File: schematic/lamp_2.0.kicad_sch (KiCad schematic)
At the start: 18 parts, among them J1 220V, J2 Disco lamp, J3 Edison lamp, Q1 BTA16, U1 EL814, U2 MOC3021, U4 TSOP31238

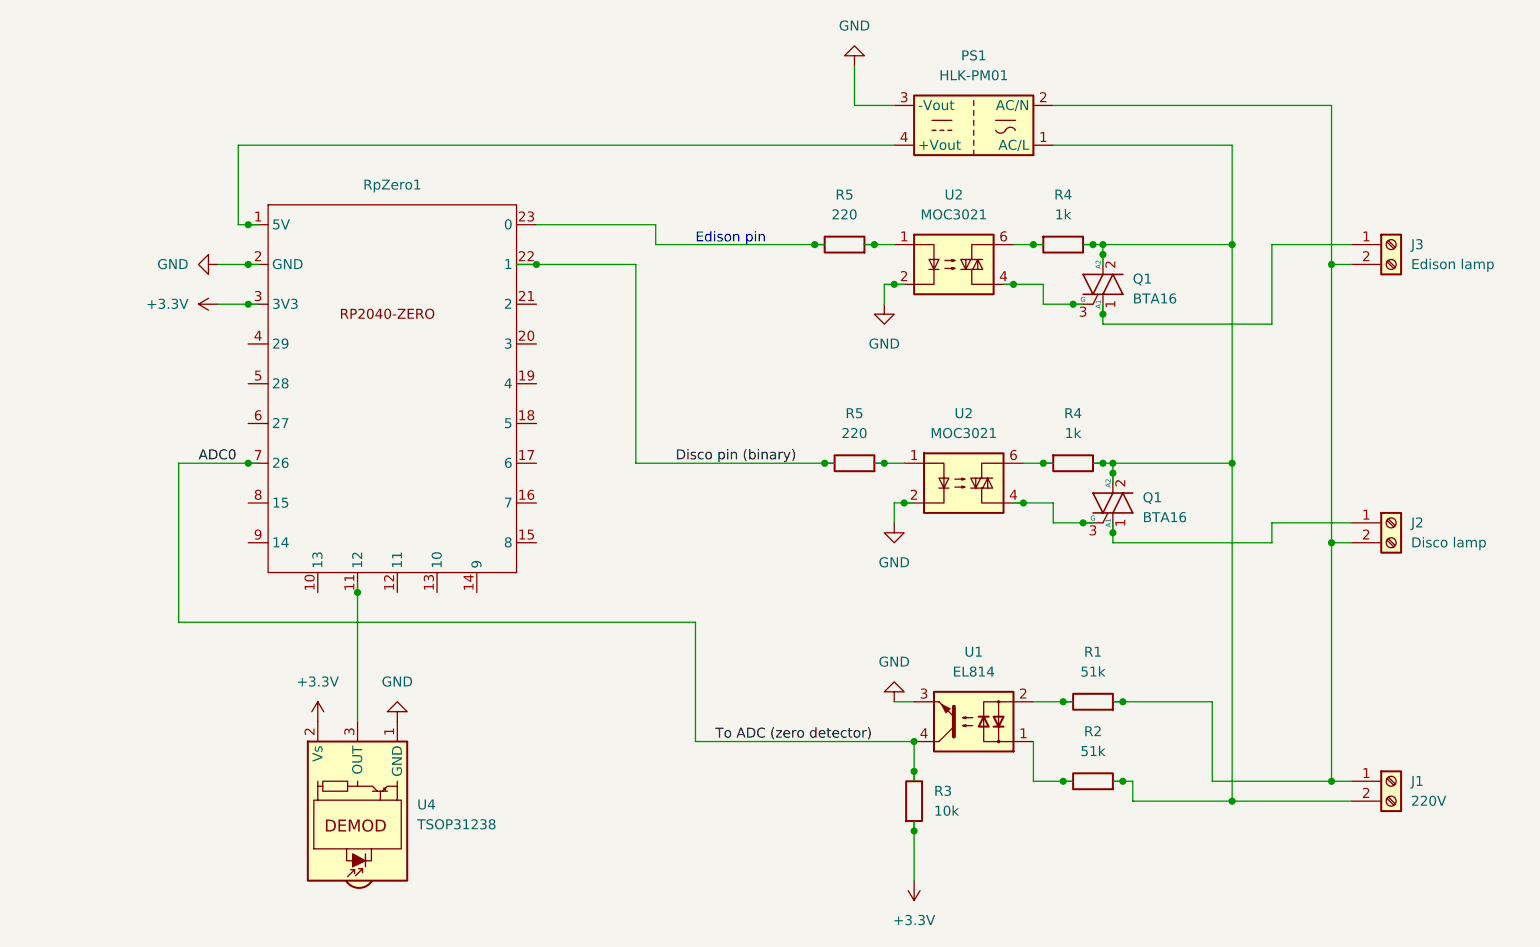
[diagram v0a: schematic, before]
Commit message: finished schema
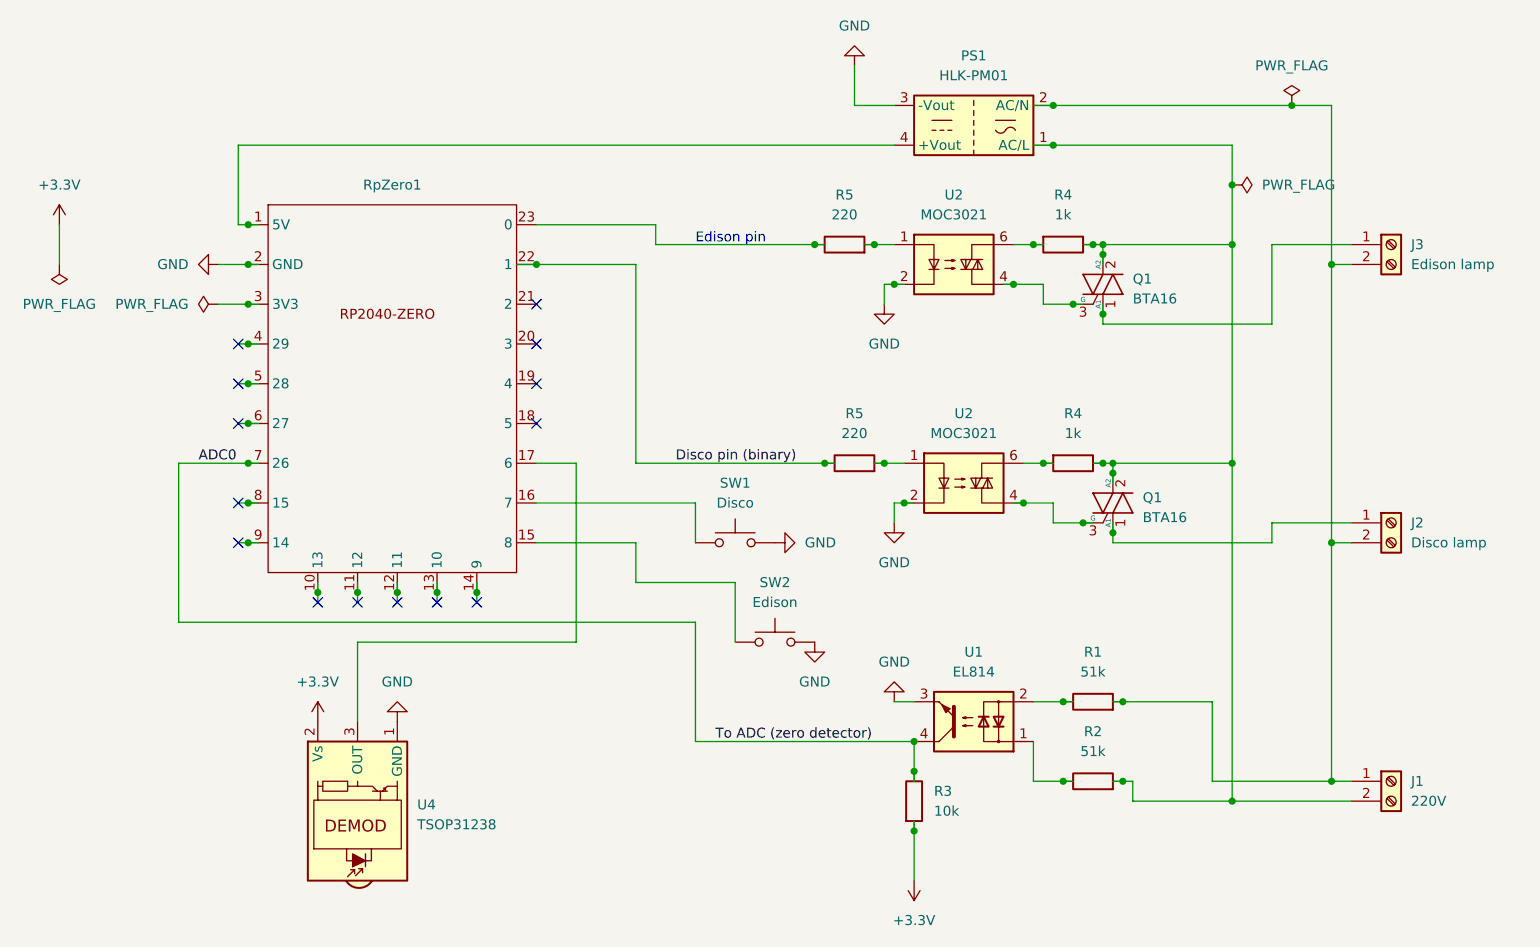
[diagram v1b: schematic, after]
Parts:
- added SW1: Disco, Connector_PinSocket_2.54mm:PinSocket_1x02_P2.54mm_Vertical, symbol Switch:SW_Push
- added SW2: Edison, Connector_PinSocket_2.54mm:PinSocket_1x02_P2.54mm_Vertical, symbol Switch:SW_Push
- J1, J2: footprint (none) -> TerminalBlock_Philmore:TerminalBlock_Philmore_TB132_1x02_P5.00mm_Horizontal
- J3: footprint (none) -> TerminalBlock_Phoenix:TerminalBlock_Phoenix_MKDS-1,5-2_1x02_P5.00mm_Horizontal
- RpZero1: footprint (none) -> kicad_library:RP-2040-FP
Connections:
- net +3.3V: no longer RpZero1.3 (3V3)
- net GND: now also SW1.2, SW2.2
- net at U4.3 (OUT): now also RpZero1.17 (6); no longer RpZero1.11 (12)
- net at RpZero1.15 (8): now also SW2.1
- net at RpZero1.16 (7): now also SW1.1
- no-connect marks 0 -> 14
